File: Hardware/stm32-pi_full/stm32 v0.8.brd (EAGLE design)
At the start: 131.4 x 105.8 mm, 256 parts, among them J1 SOLDERJUMPERNO, Q1 MMBT3906, Q2 MMBT3904, Q3 MMBT3904, U1 ESP32-WROOM-32D

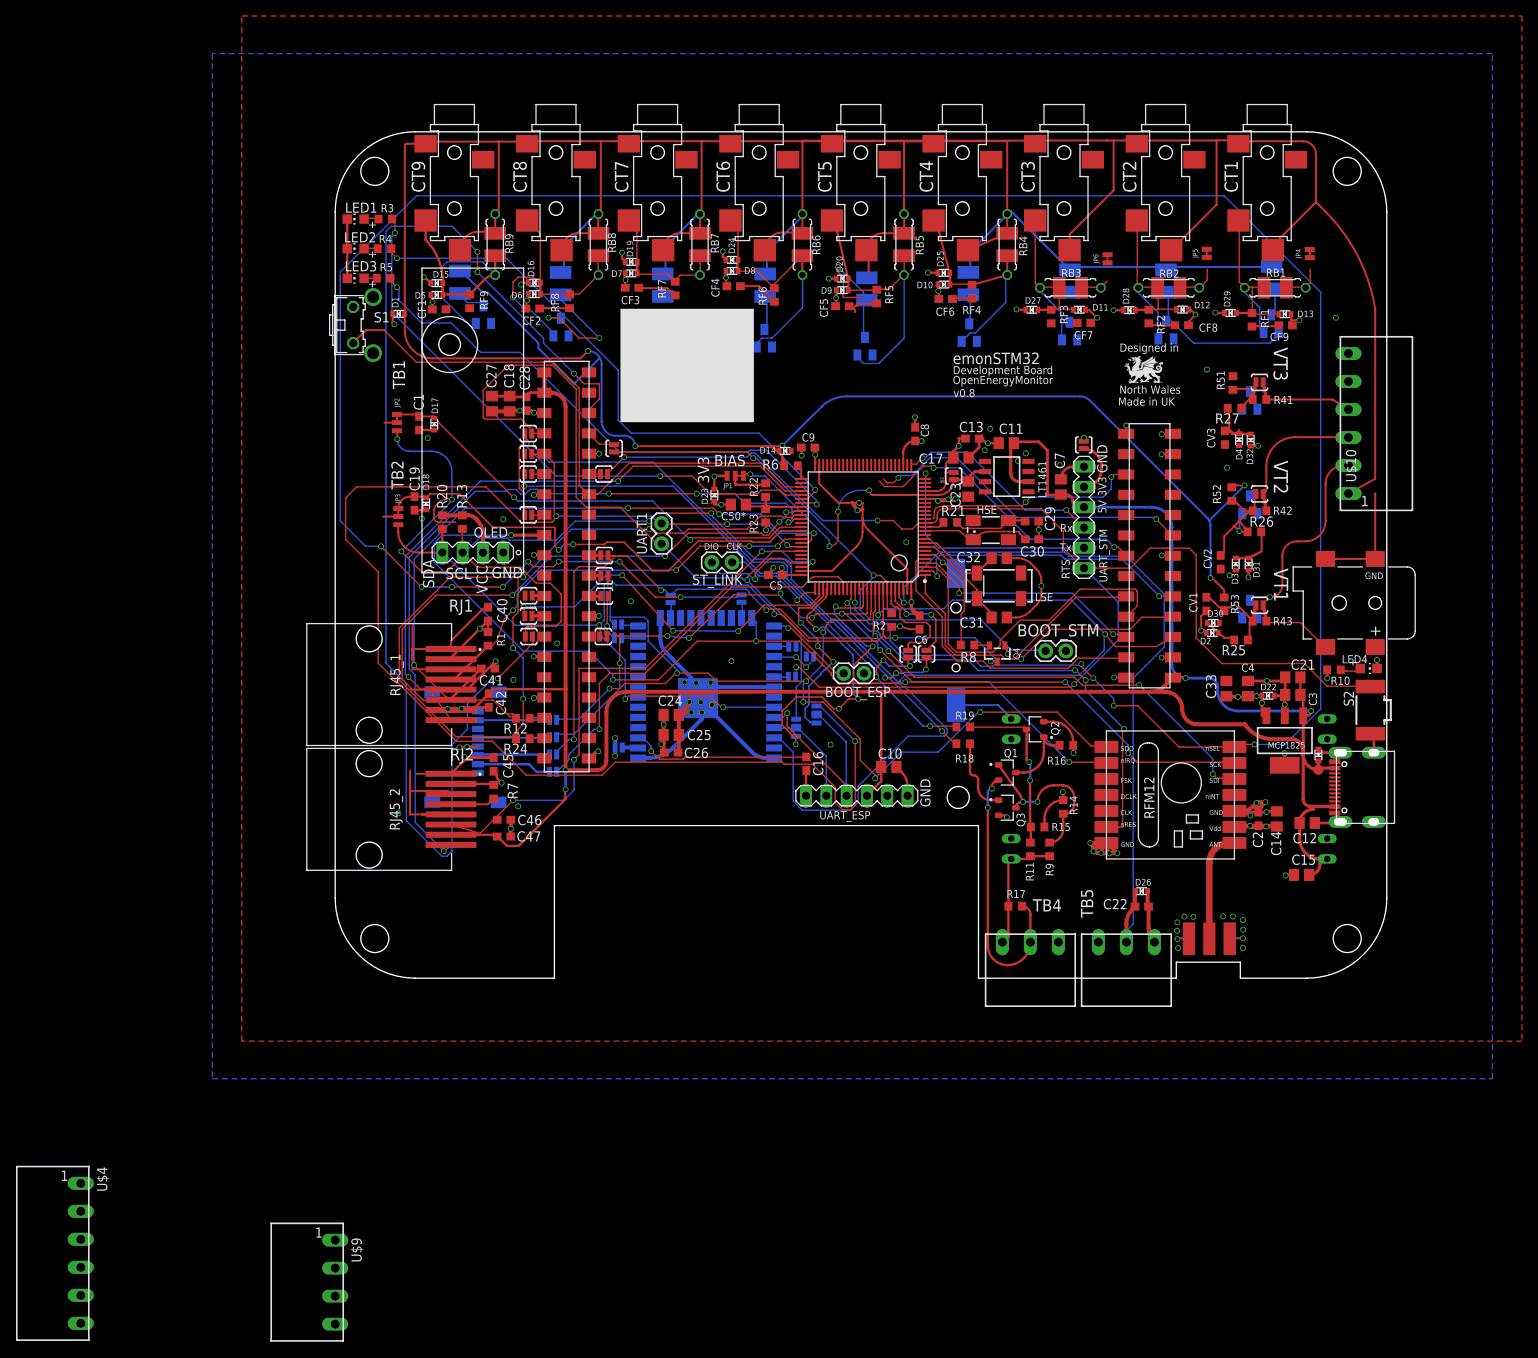
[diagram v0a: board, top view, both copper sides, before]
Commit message: update, minor board revision
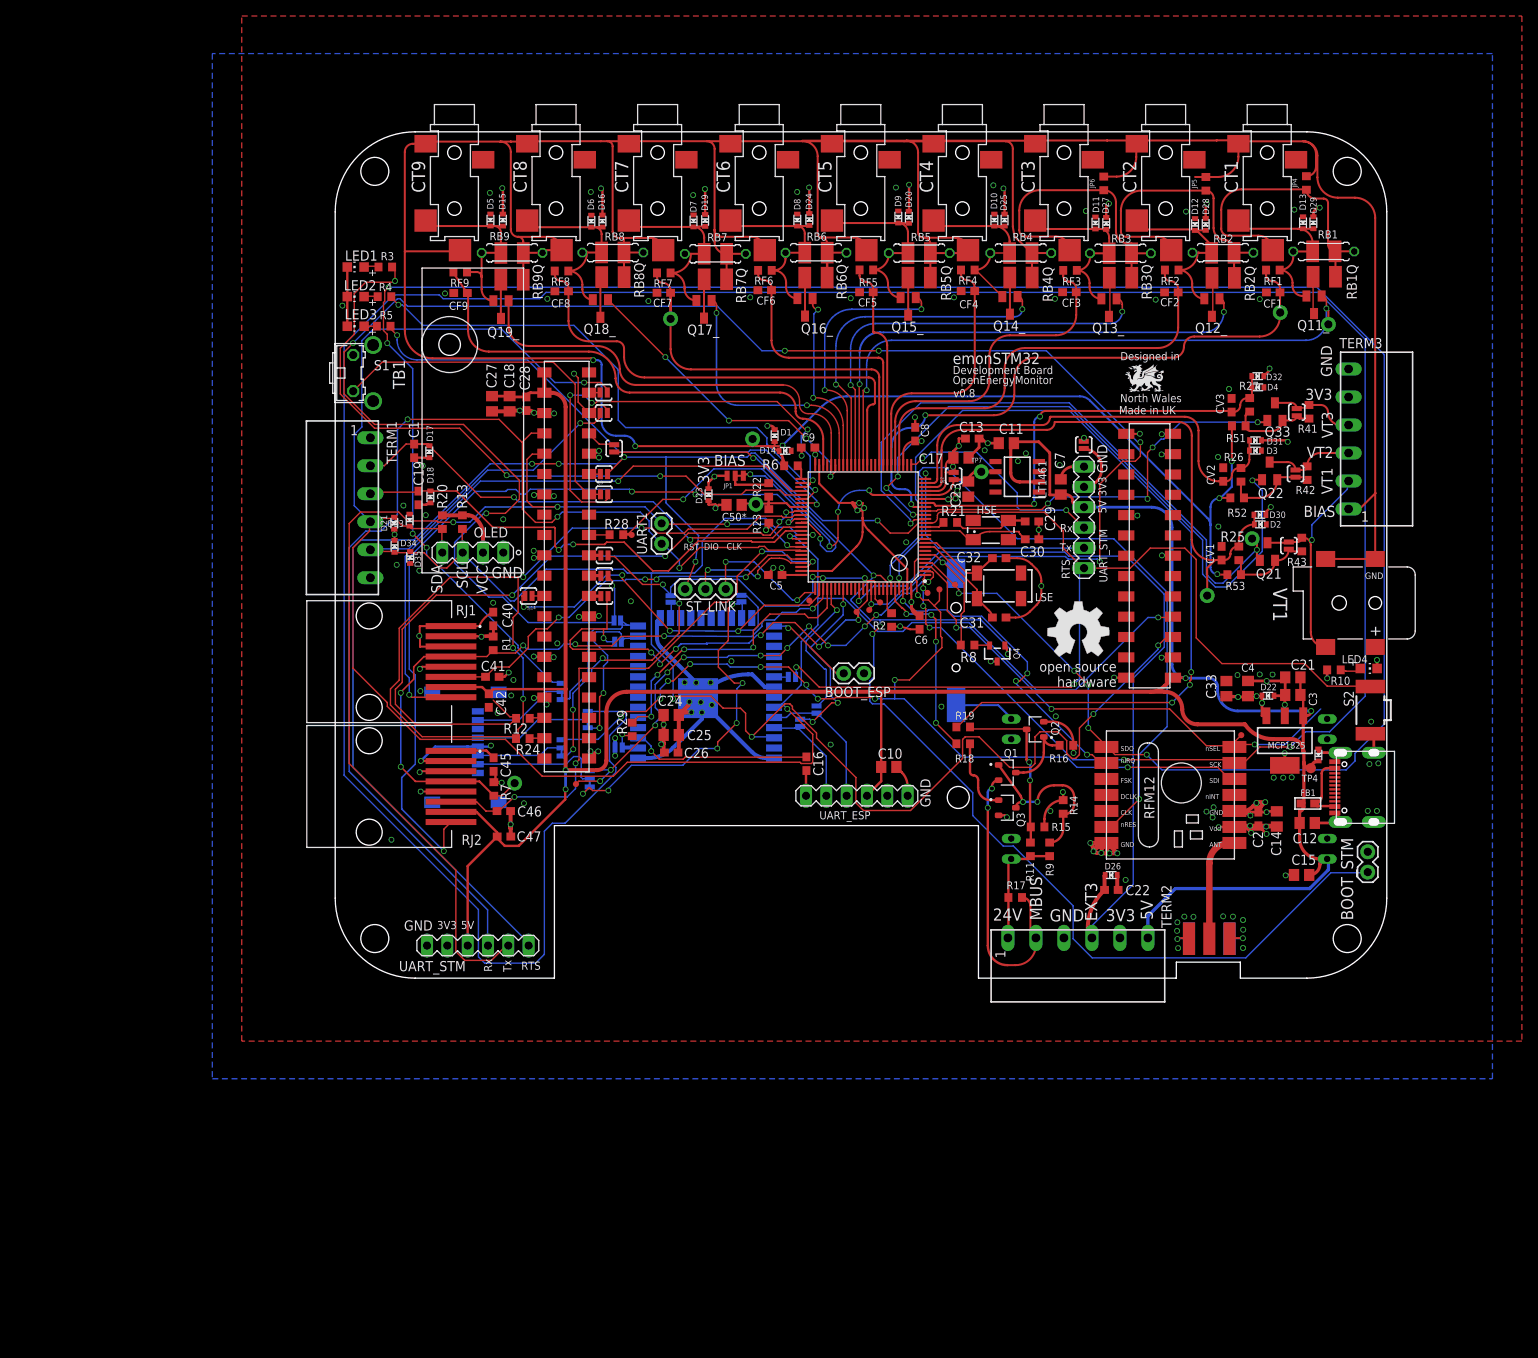
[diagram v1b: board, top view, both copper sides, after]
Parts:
- removed Q16]_: (no value), adafruit:SOT23
- removed RB1__, RB2__, RB3__, RB4__, RB5__, RB6__, RB7__, RB8__: 22r, rcl:R1210
- removed RB9__: 22r 0.1%, rcl:R1210
- removed RJ45_1, RJ45_2: 95501-6889, 95501-6889 rj45 smt:955016889
- removed SJ11, SJ12, SJ15, SJ16, SJ17, SJ18, SJ19, SJ22, SJ24, SJ28, SJ31, SJ33, SJ34, SJ8: SOLDERJUMPERNO, SparkFun:SJ_2S-NO
- removed U$10, U$4: 3.5MM_TB_X6, 3.5mm terminal block rs pro:3.5MM_X6
- removed U$5, U$6: 3.5MM_TERMINAL_BLOCK, 3.5mm terminal block rs pro:3.5MM_X3
- removed U$9: 3.5MM_TB_X4, 3.5mm terminal block rs pro:3.5MM_X4
- added D21, D33, D34, D35: ESD5Z3.3T1G, microbuilder:SOD-523
- added FB1: (no value), microbuilder:0603
- added GOLD_ORB_SM1: OSHWLOGOLOGO8MM, oshw:OSHW_8MM
- added JP7, JP8: JUMPER-SMT_3_1-NC_TRACE_SILK, SparkFun-Jumpers:SMT-JUMPER_3_1-NC_TRACE_SILK
- added Q16_: (no value), adafruit:SOT23
- added R28, R29: 10K, rcl:R0603
- added RB1Q, RB2Q, RB3Q, RB4Q, RB5Q, RB6Q, RB7Q, RB8Q: 22r, rcl:R1210
- added RB9Q: 22R 0.1%, rcl:R1210
- added RJ1, RJ2: 95501-6889, 95501-6889 rj45 smt:955016889
- added TERM1, TERM2, TERM3: 3.5MM_TB_X6, 3.5mm terminal block rs pro:3.5MM_X6
- added TP1, TP11, TP12, TP13, TP14, TP15, TP16, TP2, TP21, TP3: TEST-POINT3, SparkFun-Connectors:PAD.03X.03
- added TP10, TP17, TP18, TP19, TP20, TP5, TP6, TP7, TP9: TEST-POINTPOGO_PTH, SparkFun-Connectors:1X01_NO_SILK
- added UART_STM: (no value), con-lstb-db:MA06-1
- C29, C30: value 5nF -> 15pF
- C31, C32: value 2.2uF -> 10pF; device rcl:C0805 -> rcl:C0603
- JP2, JP3: value JUMPER-SMT_3_1-NC_TRACE_NO-SILK -> JUMPER-SMT_3_1-NC_TRACE_SILK; device SparkFun-Jumpers:SMT-JUMPER_3_1-NC_TRACE_NO-SILK -> SparkFun-Jumpers:SMT-JUMPER_3_1-NC_TRACE_SILK
- JP4, JP5, JP6: value JUMPER-SMT_2_NC_TRACE_NO-SILK -> (none); device SparkFun-Jumpers:SMT-JUMPER_2_NC_TRACE_NO-SILK -> rcl:R0603
- PCB2: value TSM-120-01-T-DV -> RPI3YA
- R12, R24: value 0R -> 10K
- RB9, RB9_: value 22r 0.1% -> 100R 0.1%
- SJ10, SJ13, SJ4, SJ9: value SOLDERJUMPERNO -> JUMPER-SMT_2_NO_SILK; device SparkFun:SJ_2S-NO -> SparkFun-Jumpers:SMT-JUMPER_2_NO_SILK
- ST_LINK: value (none) -> 455-1750-1-ND; device SparkFun:1X02 -> SparkFun-Connectors:1X03
- moved CF1 104.3 mm to (117.3, 85.7)
- moved CF9 103.2 mm to (15.7, 85.6), turned to 0 degrees
- moved CF2 79.8 mm to (104.5, 85.7)
- moved CF8 77.6 mm to (28.3, 85.9), turned to 0 degrees
- moved CF3 54.7 mm to (91.8, 85.7)
- moved CF7 52.7 mm to (41.1, 85.7), turned to 0 degrees
- moved JP2 50.6 mm to (31.8, 24.9), flipped to the bottom, turned to 270 degrees
- moved D1 49.4 mm to (54.9, 67.8), turned to 0 degrees
- moved BOOT_STM 48.8 mm to (129.1, 13.3), turned to 90 degrees
- moved SJ3 38.3 mm to (33.6, 60.5), flipped to the top, turned to 0 degrees
- moved JP3 35.4 mm to (28.3, 28.8), flipped to the bottom, turned to 270 degrees
- moved SJ26 30.5 mm to (33.6, 73.2)
- moved SJ27 29.5 mm to (33.6, 70.7)
- moved CF4 29.3 mm to (79.1, 85.9)
- moved CF6 22.6 mm to (53.7, 86.0)
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- renumbered STM32F303VE to STM32F303VET6
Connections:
- removed net +3V3_ESP: SJ23.1, U1.2
- removed net 24V: R11.2, R17.2, R9.2, U$2.OUT+, U$6.P$1
- removed net CSESP_STM32: SJ19.1, U1.27
- removed net CS_RFM69: RFM69HCW.14, SJ13.2, STM32F303VET6.86
- removed net CS_STM32: SJ19.2
- removed net DS18B20_2_RJ45: R7.1, RJ45_2.4, STM32F303VET6.81
- removed net HSPICS0: SJ13.1, U1.23
- removed net HSPID: SJ9.1, U1.16
- removed net HSPIQ: SJ4.1, U1.14
- removed net MBUS_RX: R18.2, SJ11.2, SJ33.2, SJ34.2
- removed net MBUS_RX_RPI: PCB2.P$56, SJ33.1
- removed net MBUS_TX: R19.2, SJ12.2, SJ22.2, SJ31.2
- removed net MBUS_TX_RPI: PCB2.P$52, SJ31.1
- removed net MISO: RFM69HCW.1, SJ28.2, SJ4.2, SJ6.1, STM32F303VET6.90
- removed net MOS0: Q11_.3, RB1__.2
- removed net MOSI: RFM69HCW.12, SJ16.2, SJ5.1, SJ9.2, STM32F303VET6.91
- removed net N$13: PCB2.P$66, SJ14.1
- removed net N$19: SJ8.2
- removed net N$22: PCB2.P$41
- removed net N$24: PCB2.P$57
- removed net PUSHIN_1: JP2.2, U$4.P$2
- removed net PUSHIN_1_PRE: C1.1, D17.K, JP2.3, STM32F303VET6.63
- removed net PUSHIN_2: JP3.2, U$4.P$6
- removed net PUSHIN_2_PRE: C19.1, D18.K, JP3.3, STM32F303VET6.64
- removed net PUSHIN_3: STM32F303VET6.65
- removed net PUSHIN_BYANT: C22.1, D26.K, STM32F303VET6.97, U$5.P$2
- removed net RST_RFM_ESP: SJ24.1, U1.28
- removed net SD_CS: SJ15.2, STM32F303VET6.83
- removed net SPI1_NSS: SJ14.2, STM32F303VET6.77
- removed net SPI3_CS_ESP: STM32F303VET6.84
- removed net SPI_CLK: RFM69HCW.13, SJ10.2, SJ17.2, SJ7.1, STM32F303VET6.89
- removed net UART4_RX: SJ3.2, STM32F303VET6.79
- removed net UART4_TX: SJ18.2, STM32F303VET6.78
- removed net VSIG4: EXPANSION.11
- removed net VSIG5: EXPANSION.12
- removed net VSIG6: EXPANSION.13
- removed net _AC3: R27.1, R41.2, R51.1, SJ35.1
- new net +24V: R11.2, R17.2, R9.2, TERM2.P$1, U$2.OUT+
- new net BUTTON1_STM: SJ3.2, STM32F303VET6.53
- new net ESP_PWR: R29.2, STM32F303VET6.79
- new net ESP_PWR_PRE: R29.1, SJ23.1, U1.2
- new net EXT_TERM1: C1.1, D17.K, STM32F303VET6.63, TERM1.P$2
- new net EXT_TERM2: C19.1, D18.K, STM32F303VET6.64, TERM1.P$3
- new net EXT_TERM3: C22.1, D26.K, STM32F303VET6.87, TERM2.P$4
- new net HSPI_CS0: JP2.3, SJ13.1, U1.23
- new net HSPI_ID/MOSI: JP3.3, SJ9.1, U1.16
- new net HSPI_Q/MISO: JP7.3, SJ4.1, U1.14
- new net N$20: Q11_.3, RB1Q.2
- new net N$21: Q12_.3, RB2Q.2
- new net N$23: Q13_.3, RB3Q.2
- new net RPI_PWR: R28.1, STM32F303VET6.62, TP11.P$1
- new net SPI1_CLK_SLAVE: SJ10.2, SJ7.1, STM32F303VET6.89, TP1.P$1
- new net SPI1_MISO_SLAVE: SJ4.2, SJ6.1, STM32F303VET6.90, TP2.P$1
- new net SPI1_MOSI_SLAVE: SJ5.1, SJ9.2, STM32F303VET6.91, TP3.P$1
- new net SPI1_NSS_SLAVE: SJ13.2, SJ14.2, STM32F303VET6.77, TP21.P$1
- new net SPI4_CLK_MASTER: JP8.1, RFM69HCW.13, STM32F303VET6.1, TP12.P$1
- new net SPI4_CS_RFM69_MASTER: RFM69HCW.14, STM32F303VET6.3, TP14.P$1
- new net SPI4_CS_SDCARD_MASTER: JP2.1, STM32F303VET6.2, TP13.P$1
- new net SPI4_MISO_MASTER: JP7.1, RFM69HCW.1, STM32F303VET6.4, TP15.P$1
- new net SPI4_MOSI_MASTER: JP3.1, RFM69HCW.12, STM32F303VET6.5, TP16.P$1
- new net UART5_RX: SJ20.1, STM32F303VET6.83
- new net UART5_TX: SJ21.1, STM32F303VET6.80
- net +3V3: now also D21.K, D34.K, RJ1.2, RJ2.2, TERM1.P$1, TERM2.P$5, TERM3.P$5, UART_STM.2; no longer RJ45_1.2, RJ45_2.2, U$10.P$5, U$4.P$3, U$5.P$1
- net +5V: now also FB1.2, RJ1.7, RJ2.7, TERM2.P$6, UART_STM.3; no longer RJ45_1.7, RJ45_2.7, USB-C.A4/B9, USB-C.B4/A9
- net AC1: now also TERM3.P$2; no longer U$10.P$2
- net AC1_MOS: no longer CV1.1
- net AC2: now also TERM3.P$3; no longer U$10.P$3
- net AC2_MOS: no longer CV2.1
- net AC3: now also TERM3.P$4; no longer U$10.P$4
- net AC3_MOS: now also R27.1, R41.2, R51.1, SJ35.1
- net ADC_2_RJ45IN: now also RJ2.8; no longer RJ45_2.8
- net ADC_RJ45IN: now also RJ1.8; no longer RJ45_1.8
- net BIAS: now also RB4Q.1, RB5Q.1, RB6Q.1, RB7Q.1, RB8Q.1, RB9Q.1, TERM3.P$1, TP5.1; no longer CT1.P$4, CT2.P$4, CT3.P$4, RB1__.1, RB2__.1, RB3__.1, RB4__.1, RB5__.1, RB6__.1, RB7__.1, RB8__.1, RB9__.1, U$10.P$1
- net BIAS_IN: now also TP10.1
- net BUTTON1: now also SJ3.1; no longer STM32F303VET6.53
- net CT1: now also CF1.2, TP18.1; no longer CF9.2, STM32F303VET6.35
- net CT2: now also CF2.2; no longer CF8.2, STM32F303VET6.36
- net CT3: now also CF3.2; no longer CF7.2
- net CT4: now also CF4.2; no longer CF6.2
- net CT6: now also CF6.2; no longer CF4.2
- net CT7: now also CF7.2, TP19.1; no longer CF3.2
- net CT8: now also CF8.2; no longer CF2.2
- net CT9: now also CF9.2; no longer CF1.2
- net DIO0_RFM: now also STM32F303VET6.98; no longer PCB2.P$58, STM32F303VET6.88, U1.24
- net DS18B20_RJ45: now also R7.1, RJ1.4, RJ2.4, STM32F303VET6.78, TP9.1; no longer RJ45_1.4, STM32F303VET6.66
- net GND: now also D33.A, D35.A, RJ1.1, RJ1.3, RJ1.5, RJ2.1, RJ2.3, RJ2.5, TERM1.P$6, TERM2.P$3, TERM3.P$6, UART_STM.1; no longer RJ45_1.1, RJ45_1.3, RJ45_1.5, RJ45_2.1, RJ45_2.3, RJ45_2.5, U$10.P$6, U$4.P$1, U$4.P$4, U$4.P$5, U$5.P$3, U$6.P$3
- net HSPI_CLK: now also JP8.3
- net IO2_EX: no longer STM32F303VET6.98
- net IO3_EX: no longer STM32F303VET6.1
- net IO4_EX: no longer STM32F303VET6.2
- net IO5_EX: no longer STM32F303VET6.3
- net IO6_EX: no longer STM32F303VET6.4
- net IO7_EX: no longer STM32F303VET6.5
- net MBUS_I/O: now also TERM2.P$2; no longer U$6.P$2
- net MOS1: now also TP17.1; no longer Q12_.3, RB2__.2
- net MOS2: no longer Q13_.3, RB3__.2
- net MOS6: now also Q16_.1; no longer Q16]_.1
- net N$11: now also SJ14.1; no longer SJ8.1
- net N$18: now also PCB2.P$57, R28.2; no longer STM32F303VET6.80
- net N$26: now also CT1.P$4, RB1Q.1
- net N$27: now also CT2.P$4, RB2Q.1
- net N$28: now also CT3.P$4, RB3Q.1
- net N$37: now also RB4Q.2; no longer RB4__.2
- net N$38: now also Q16_.2; no longer Q16]_.2
- net N$45: now also RB9Q.2; no longer RB9__.2
- net N$46: now also RB8Q.2; no longer RB8__.2
- net N$47: now also RB5Q.2; no longer RB5__.2
- net N$48: now also Q16_.3, RB6Q.2; no longer Q16]_.3, RB6__.2
- net N$49: now also RB7Q.2; no longer RB7__.2
- net N$7: now also FB1.1, USB-C.A4/B9, USB-C.B4/A9; no longer STM32F303VET6.87
- net NRST_STM: now also ST_LINK.3, UART_STM.6
- net PULSE1_RJ45: now also RJ1.6, STM32F303VET6.71; no longer RJ45_1.6, STM32F303VET6.67
- net PULSE_2_RJ45: now also RJ2.6; no longer RJ45_2.6
- net RST_RFM: now also STM32F303VET6.97; no longer SJ24.2, STM32F303VET6.85
- net RXD0_ESP: no longer SJ18.1
- net SCL: now also D34.A, D35.K, STM32F303VET6.65, TERM1.P$5; no longer JP2.1, STM32F303VET6.92
- net SDA: now also D21.A, D33.K, STM32F303VET6.66, TERM1.P$4; no longer JP3.1, STM32F303VET6.93
- net SD_CLK: now also JP8.2; no longer SJ17.1
- net SD_CS_: now also JP2.2; no longer SJ15.1
- net SD_MISO: now also JP7.2; no longer SJ28.1
- net SD_MOSI: now also JP3.2; no longer SJ16.1
- net TXD0_ESP: no longer SJ3.1
- net UART1_RX: now also UART_STM.4; no longer SJ11.1, SJ20.1
- net UART1_TX: now also UART_STM.5; no longer SJ12.1, SJ21.1
- net USART3_RX: now also R19.2; no longer SJ22.1
- net USART3_TX: now also R18.2; no longer SJ34.1
- net VMOS1: now also TP6.1
- net VREF+: now also TP7.1
- net VSIG1: now also CV1.1, TP20.1
- net VSIG2: now also CV2.1
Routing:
- net SPI4_CLK_MASTER: track 0.00 -> 383.8 mm, vias 0 -> 5
- net CS_RFM69: track 343.9 -> 0.00 mm, vias 13 -> 0
- net SPI4_MISO_MASTER: track 0.00 -> 308.5 mm, vias 0 -> 9
- net SPI1_MISO_SLAVE: track 0.00 -> 238.1 mm, vias 0 -> 8
- net SCL_: track 155.1 -> 9.02 mm, vias 4 -> 1
- net MOSI: track 128.3 -> 0.00 mm, vias 7 -> 0
- net MISO: track 122.6 -> 0.00 mm, vias 8 -> 0
- net SPI_CLK: track 121.5 -> 0.00 mm, vias 10 -> 0
- net SPI4_MOSI_MASTER: track 0.00 -> 121.4 mm, vias 0 -> 11
- net NRST_STM: track 175.9 -> 288.0 mm, vias 4 -> 7
- net EXT_TERM3: track 0.00 -> 99.7 mm, vias 0 -> 1
- net DIO0_RFM: track 137.6 -> 39.4 mm, vias 7 -> 4
- net USART3_RX: track 13.6 -> 111.8 mm, vias 0 -> 4
- net PUSHIN_BYANT: track 92.5 -> 0.00 mm, vias 1 -> 0
- net BOOT0: track 75.3 -> 166.8 mm, vias 2 -> 4
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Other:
- board text added: "24V"
- board text added: "EXT3"
- board text added: "MBUS"
- board text added: "RST"
- board text added: "TP4"
- board text removed: "RJ1"
- board text removed: "RJ2"
- board text removed: "TB2"
- board text removed: "TB4"
- board text removed: "TB5"
